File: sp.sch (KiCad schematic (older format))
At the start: 90 parts, among them J301 Conn_ARM_JTAG_SWD_10, J302 HOST_UART, J303 AUX_HDR_J, J304 AUX_HDR_G, SW301 RESET, SW302 BOOT0, U301 STM32H753BITx, U302 MAX13235EET, Y301 8 MHz / H130A-8.000-8-2030, Y302 32.768kHz / FC-135 32.7680KA-A

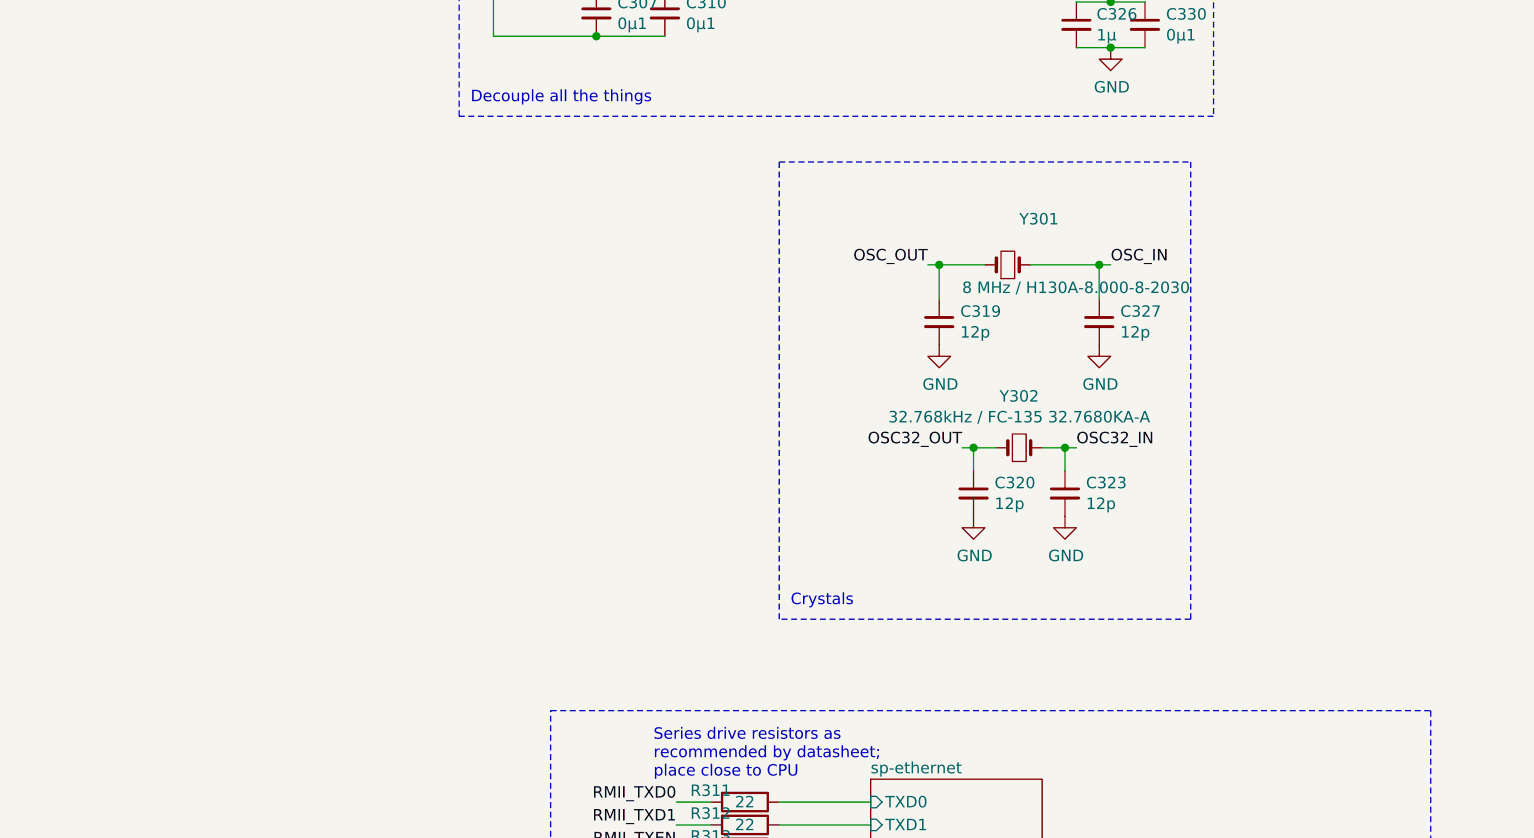
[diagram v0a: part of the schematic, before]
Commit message: sp: recalculate and document crystal load capacitor constraints
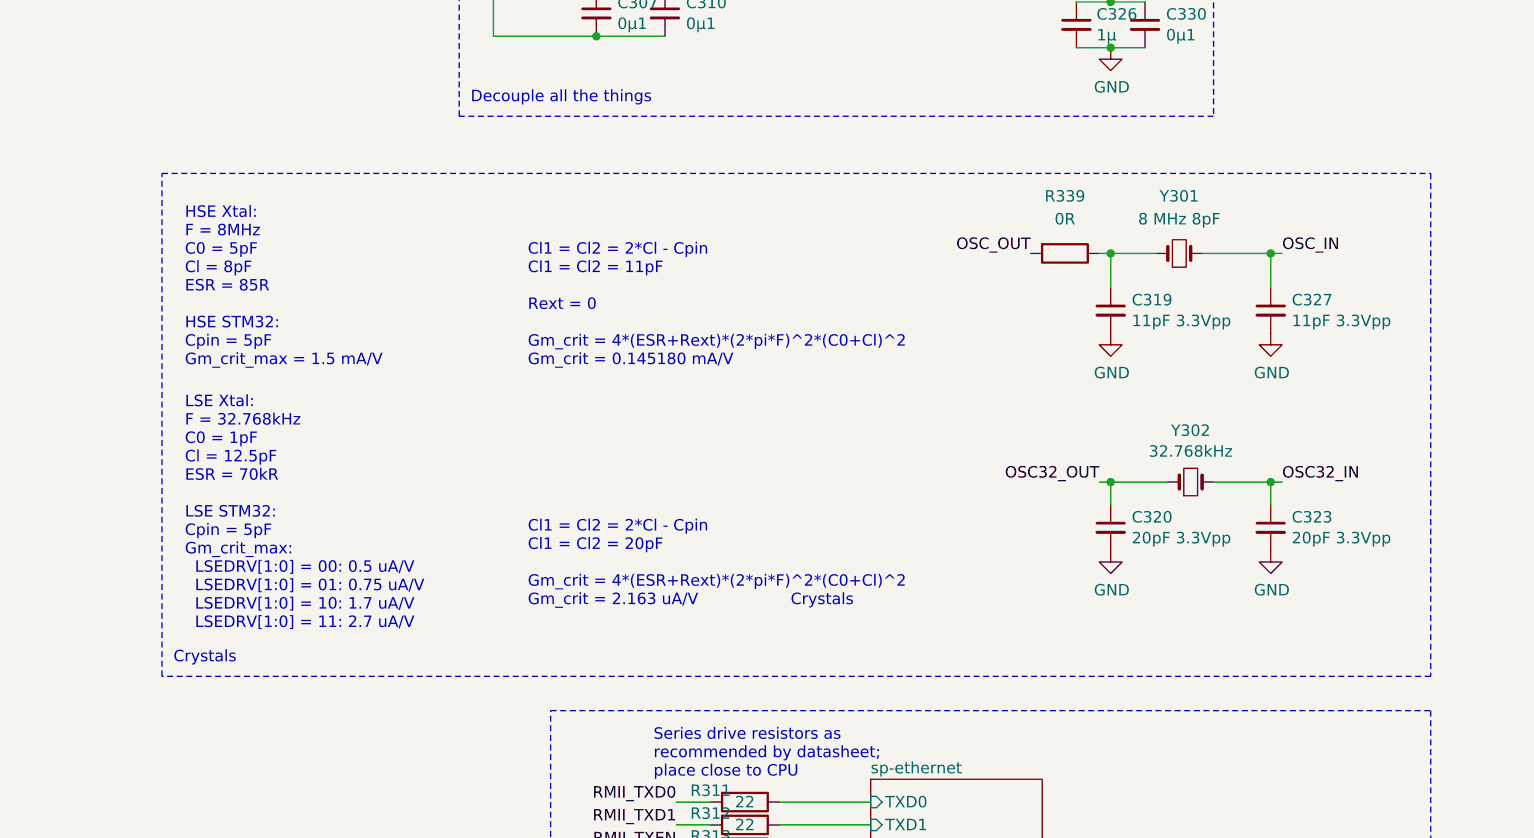
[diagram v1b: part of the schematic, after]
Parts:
- added R339: 0R, symbol Device:R
- C319, C327: value 12p -> 11pF 3.3Vpp
- C320, C323: value 12p -> 20pF 3.3Vpp
- Y301: value 8 MHz / H130A-8.000-8-2030 -> 8 MHz 8pF
- Y302: value 32.768kHz / FC-135 32.7680KA-A -> 32.768kHz
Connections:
- net OSC_OUT: now also R339.2; no longer C319.1, Y301.1
- new net: C319.1, R339.1, Y301.1
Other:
- note added: "Cl1 = Cl2 = 2*Cl - Cpin\nCl1 = Cl2 = 11pF\n\nRext = 0\n\nGm_crit = 4*(ESR+Rext)*(2*pi*F)^2*(C0+Cl)^2\nGm_crit = 0.145180 mA/V"
- note added: "Cl1 = Cl2 = 2*Cl - Cpin\nCl1 = Cl2 = 20pF\n\nGm_crit = 4*(ESR+Rext)*(2*pi*F)^2*(C0+Cl)^2\nGm_crit = 2.163 uA/V"
- note added: "HSE Xtal:\nF = 8MHz\nC0 = 5pF\nCl = 8pF\nESR = 85R\n\nHSE STM32:\nCpin = 5pF\nGm_crit_max = 1.5 mA/V"
- note added: "LSE Xtal:\nF = 32.768kHz\nC0 = 1pF\nCl = 12.5pF\nESR = 70kR\n\nLSE STM32:\nCpin = 5pF\nGm_crit_max:\n LSEDRV[1:0] = 00: 0.5 uA/V\n LSEDRV[1:0] = 01: 0.75 uA/V\n LSEDRV[1:0] = 10: 1.7 uA/V\n LSEDRV[1:0] = 11: 2.7 uA/V\n"
- moved on the sheet: C319, C320, C323, C327, Y301, Y302
